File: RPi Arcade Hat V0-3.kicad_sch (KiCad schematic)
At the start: 75 parts, among them J1 Raspberry_Pi_2_3, J10 Coin/Note Input, J11 +24V IN, J12 +12V OUT, J13 Player 1, J14 Player 2, J15 Player 3, J16 Player 4, J17 ICSP, J18 Program MCU, J19 Graphics LCD, J2 Player 1, J20 Channel 4, J21 Channel 3, J22 Channel 2, J23 Channel 1, J24 CCard Input, J3 Player 2, J4 Spares, J5 Player 3, J6 Player 4, J7 +24V OUT, J8 Neo Pixel Data, J9 Note Acceptor, Q16 BC847, Q4 BC847, Q5 BC847, Q6 BC847, Q7 BC847, U1 ATmega328P-A, U2 SN74HC04N, U3 LM2595S-12, Y1 16MHz Crystal

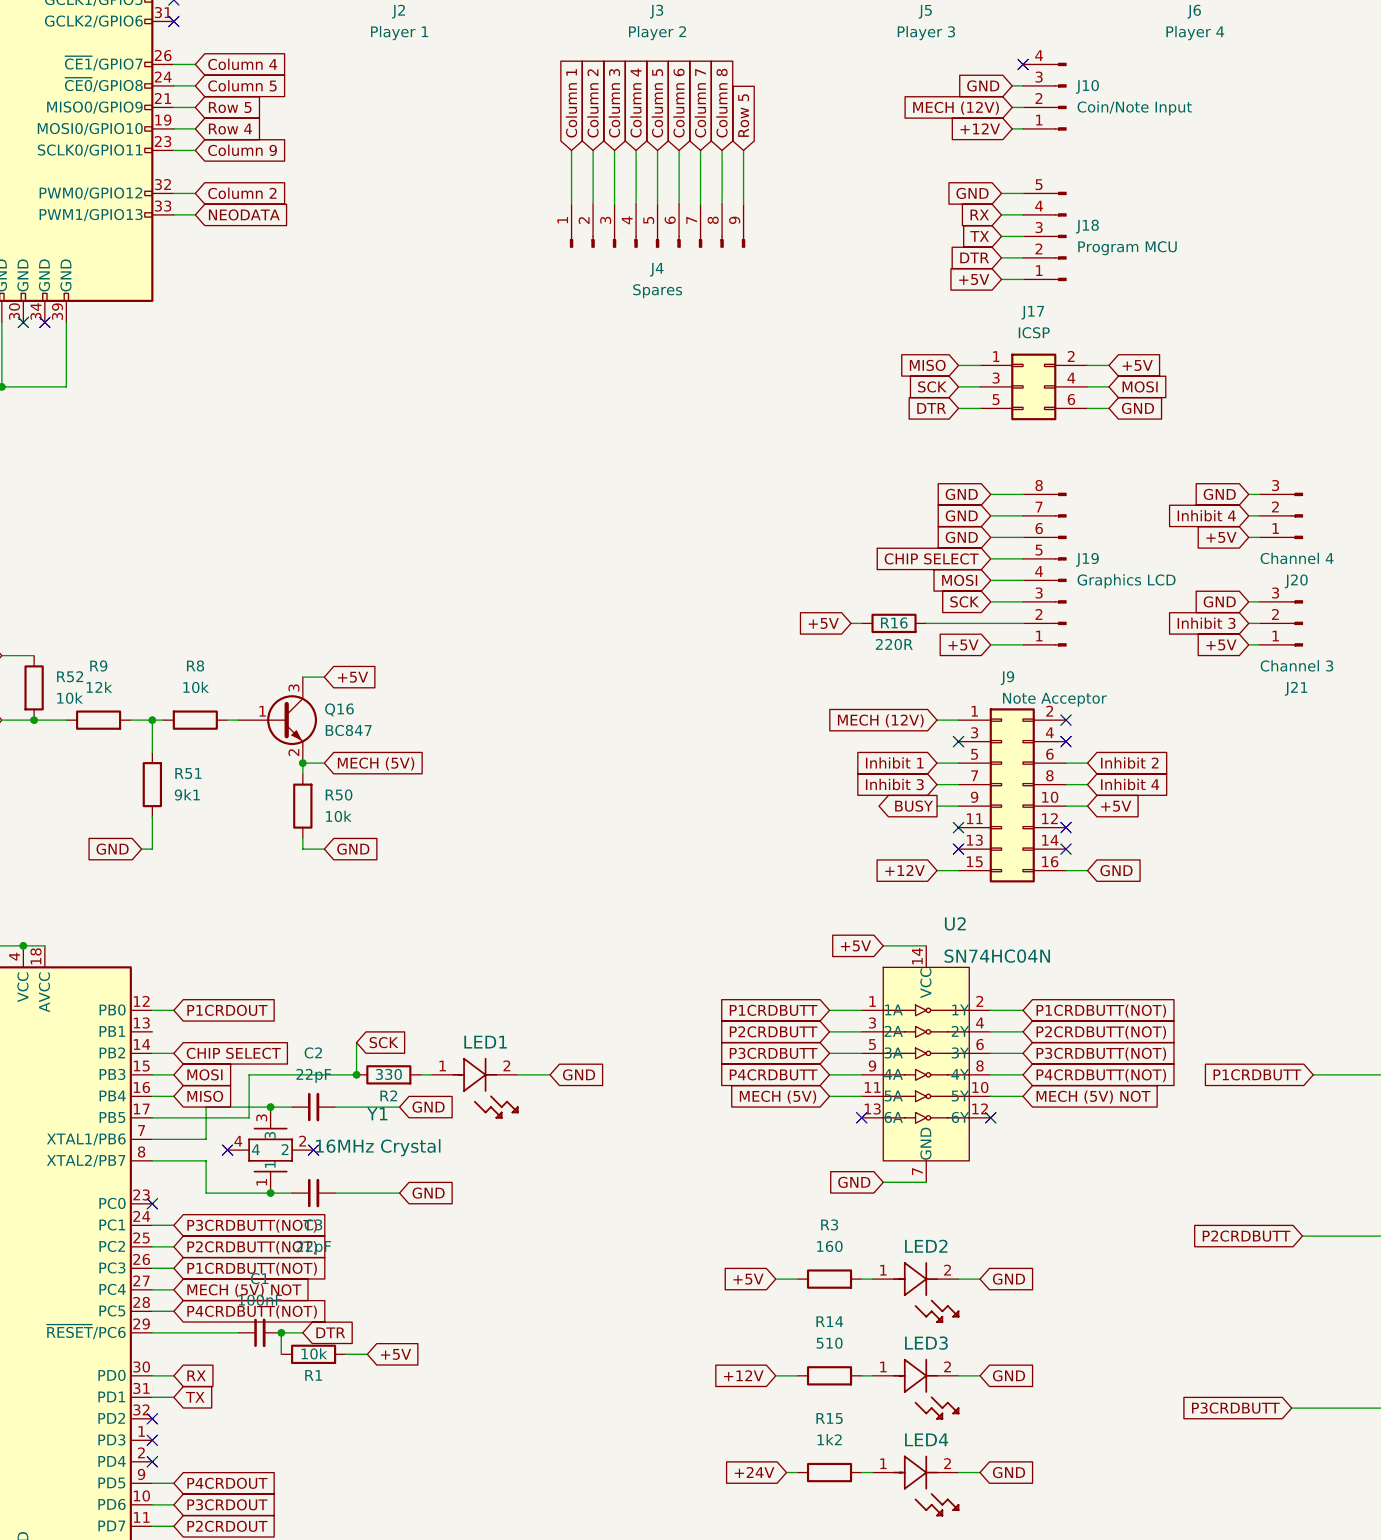
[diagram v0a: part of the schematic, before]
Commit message: Added Arduino Code
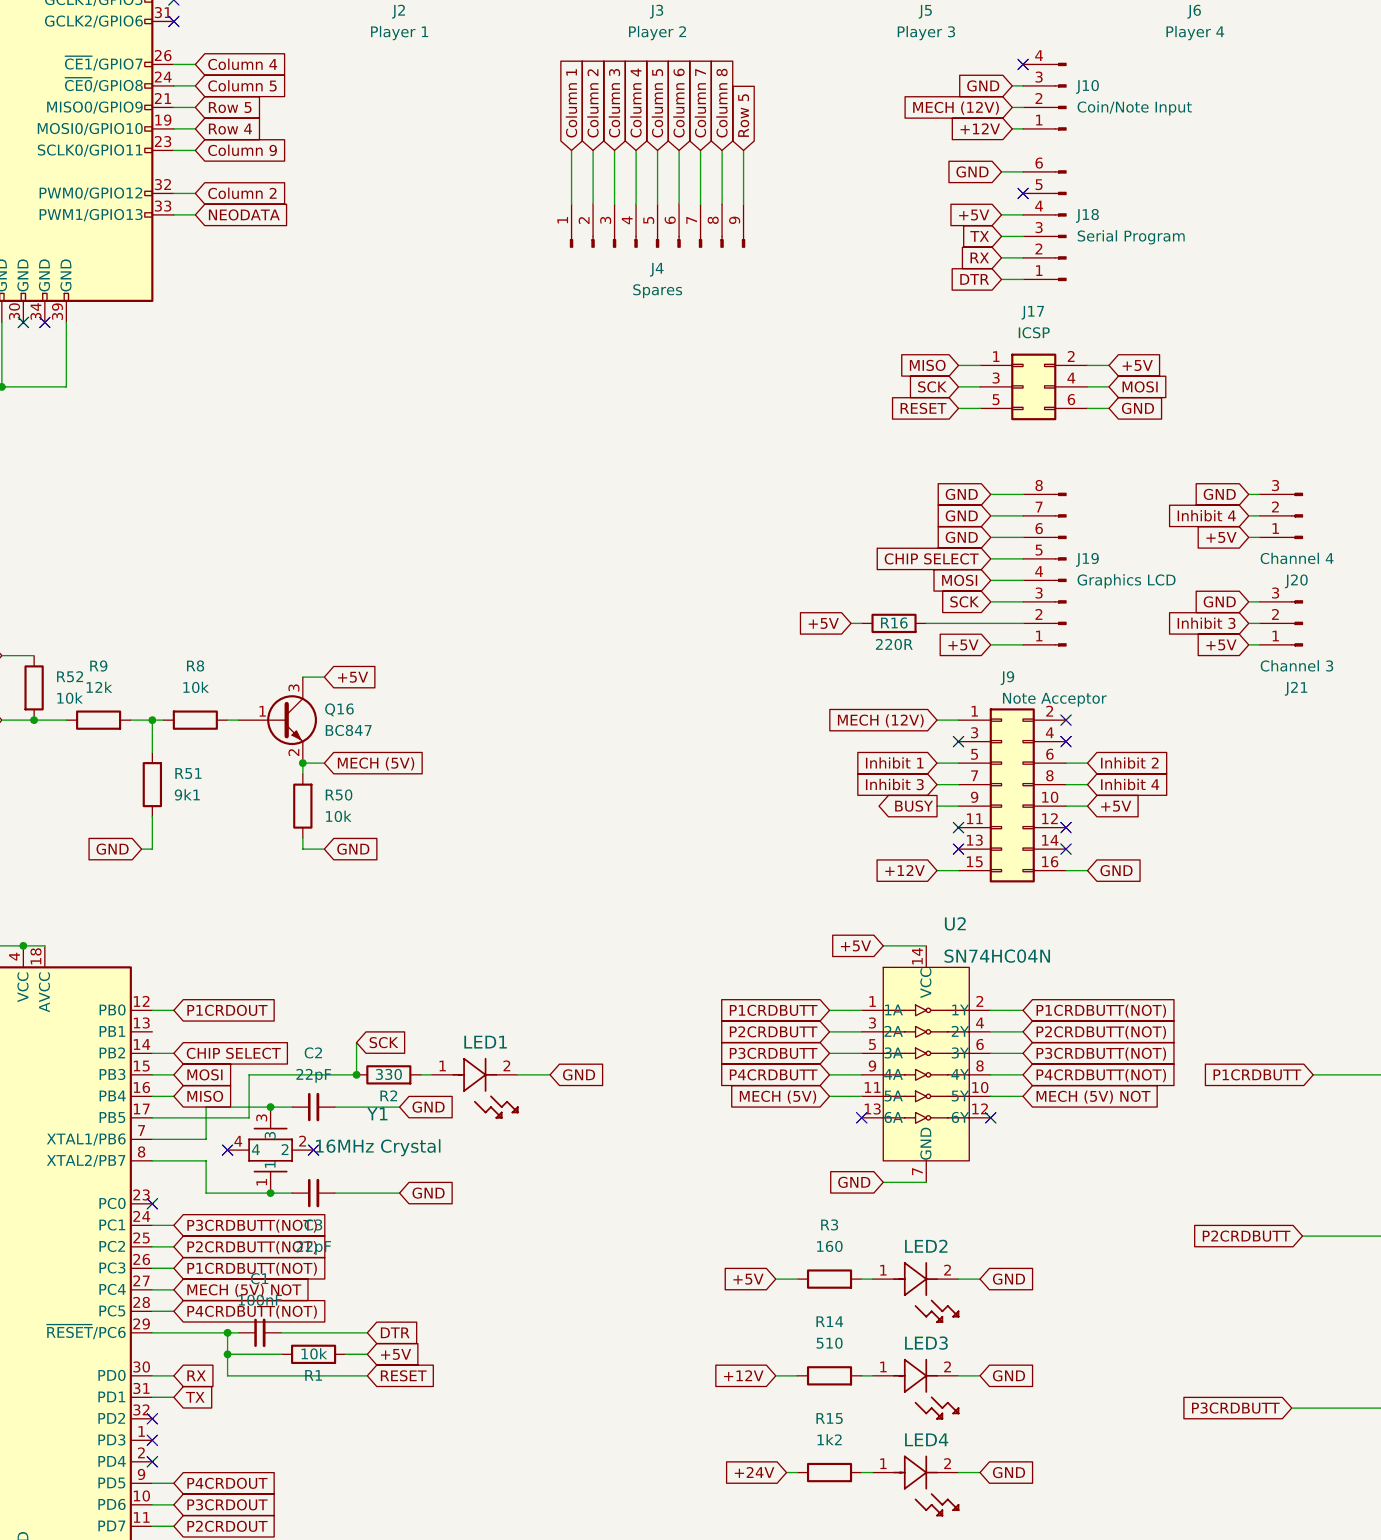
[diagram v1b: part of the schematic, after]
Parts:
- removed J18: Program MCU, Connector_PinHeader_2.54mm:PinHeader_1x05_P2.54mm_Vertical, symbol Connector:Conn_01x05_Male
- added J18: Serial Program, Connector_PinHeader_2.54mm:PinHeader_1x06_P2.54mm_Vertical, symbol Connector:Conn_01x06_Pin
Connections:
- net +5V: now also J18.4 (Pin_4)
- net DTR: now also J18.1 (Pin_1); no longer J17.5 (Pin_5), R1.1
- net GND: now also J18.6 (Pin_6)
- net RX: now also J18.2 (Pin_2)
- net TX: now also J18.3 (Pin_3)
- net RESET: now reaches C1.1, U1.29 (~{RESET}/PC6)
- net RESET: now also J17.5 (Pin_5), R1.1
- no-connect marks 36 -> 37
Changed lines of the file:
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@@
   (junction (at 63.5 257.81) (diameter 0) (color 0 0 0 0)
   )
+  (junction (at 74.93 204.47) (diameter 0) (color 0 0 0 0)
+  )
   (junction (at 83.82 137.16) (diameter 0) (color 0 0 0 0)
   )
   (junction (at 40.64 92.71) (diameter 0) (color 0 0 0 0)
   )
+  (junction (at 74.93 207.01) (diameter 0) (color 0 0 0 0)
+  )
   (junction (at 63.5 265.43) (diameter 0) (color 0 0 0 0)
   )
@@
   (junction (at 26.67 252.73) (diameter 0) (color 0 0 0 0)
   )
-  (junction (at 81.28 204.47) (diameter 0) (color 0 0 0 0)
-  )
   (junction (at 227.33 213.36) (diameter 0) (color 0 0 0 0)
   )
@@
   (no_connect (at 50.8 85.09))
   (no_connect (at 35.56 171.45))
+  (no_connect (at 168.91 69.85))
   (no_connect (at 45.72 85.09))
   (no_connect (at 161.29 134.62))
@@
     (stroke (width 0) (type default))
   )
-  (wire (pts (xy 166.37 72.39) (xy 168.91 72.39))
-    (stroke (width 0) (type default))
-  )
   (wire (pts (xy 149.86 198.12) (xy 151.13 198.12))
     (stroke (width 0) (type default))
@@
     (stroke (width 0) (type default))
   )
-  (wire (pts (xy 166.37 77.47) (xy 168.91 77.47))
-    (stroke (width 0) (type default))
-  )
   (wire (pts (xy 165.1 110.49) (xy 168.91 110.49))
     (stroke (width 0) (type default))
@@
     (stroke (width 0) (type default))
   )
+  (wire (pts (xy 74.93 209.55) (xy 74.93 207.01))
+    (stroke (width 0) (type default))
+  )
   (wire (pts (xy 248.92 190.5) (xy 247.65 190.5))
     (stroke (width 0) (type default))
   )
-  (wire (pts (xy 166.37 69.85) (xy 168.91 69.85))
+  (wire (pts (xy 166.37 67.31) (xy 168.91 67.31))
     (stroke (width 0) (type default))
   )
@@
     (stroke (width 0) (type default))
   )
+  (wire (pts (xy 74.93 204.47) (xy 76.2 204.47))
+    (stroke (width 0) (type default))
+  )
   (wire (pts (xy 147.32 34.29) (xy 147.32 40.64))
     (stroke (width 0) (type default))
@@
     (stroke (width 0) (type default))
   )
+  (wire (pts (xy 81.28 207.01) (xy 74.93 207.01))
+    (stroke (width 0) (type default))
+  )
   (wire (pts (xy 226.06 237.49) (xy 248.92 237.49))
     (stroke (width 0) (type default))
@@
     (stroke (width 0) (type default))
   )
-  (wire (pts (xy 66.04 204.47) (xy 76.2 204.47))
+  (wire (pts (xy 66.04 204.47) (xy 74.93 204.47))
     (stroke (width 0) (type default))
   )
@@
     (stroke (width 0) (type default))
   )
+  (wire (pts (xy 74.93 207.01) (xy 74.93 204.47))
+    (stroke (width 0) (type default))
+  )
   (wire (pts (xy 25.4 69.85) (xy 27.94 69.85))
     (stroke (width 0) (type default))
@@
     (stroke (width 0) (type default))
   )
+  (wire (pts (xy 166.37 74.93) (xy 168.91 74.93))
+    (stroke (width 0) (type default))
+  )
   (wire (pts (xy 231.14 171.45) (xy 231.14 173.99))
     (stroke (width 0) (type default))
@@
     (stroke (width 0) (type default))
   )
-  (wire (pts (xy 81.28 204.47) (xy 81.28 207.01))
-    (stroke (width 0) (type default))
-  )
   (wire (pts (xy 165.1 171.45) (xy 168.91 171.45))
     (stroke (width 0) (type default))
@@
     (stroke (width 0) (type default))
   )
+  (wire (pts (xy 166.37 72.39) (xy 168.91 72.39))
+    (stroke (width 0) (type default))
+  )
   (wire (pts (xy 161.29 149.86) (xy 158.75 149.86))
     (stroke (width 0) (type default))
@@
     (stroke (width 0) (type default))
   )
+  (wire (pts (xy 166.37 80.01) (xy 168.91 80.01))
+    (stroke (width 0) (type default))
+  )
   (wire (pts (xy 115.57 34.29) (xy 115.57 40.64))
     (stroke (width 0) (type default))
@@
     (stroke (width 0) (type default))
   )
-  (wire (pts (xy 66.04 166.37) (xy 68.58 166.37))
+  (wire (pts (xy 166.37 77.47) (xy 168.91 77.47))
     (stroke (width 0) (type default))
   )
-  (wire (pts (xy 166.37 80.01) (xy 168.91 80.01))
+  (wire (pts (xy 66.04 166.37) (xy 68.58 166.37))
     (stroke (width 0) (type default))
   )
@@
     (stroke (width 0) (type default))
   )
-  (wire (pts (xy 81.28 204.47) (xy 83.82 204.47))
+  (wire (pts (xy 81.28 204.47) (xy 91.44 204.47))
     (stroke (width 0) (type default))
   )
@@
     (stroke (width 0) (type default))
   )
+  (wire (pts (xy 91.44 209.55) (xy 74.93 209.55))
+    (stroke (width 0) (type default))
+  )
   (wire (pts (xy 189.23 34.29) (xy 189.23 40.64))
     (stroke (width 0) (type default))
@@
     (stroke (width 0) (type default))
   )
-  (wire (pts (xy 166.37 74.93) (xy 168.91 74.93))
-    (stroke (width 0) (type default))
-  )
   (wire (pts (xy 87.63 177.8) (xy 95.25 177.8))
     (stroke (width 0) (type default))
@@
     )
   )
-  (global_label "DTR" (shape input) (at 161.29 95.25 180) (fields_autoplaced)
+  (global_label "RESET" (shape input) (at 161.29 95.25 180) (fields_autoplaced)
     (effects (font (size 1.27 1.27)) (justify right))
-    (property "Intersheetrefs" "${INTERSHEET_REFS}" (at 155.3693 95.1706 0)
+    (property "Intersheetrefs" "${INTERSHEET_REFS}" (at 152.5597 95.25 0)
       (effects (font (size 1.27 1.27)) (justify right) hide)
     )
@@
     )
   )
-  (global_label "DTR" (shape input) (at 83.82 204.47 0) (fields_autoplaced)
+  (global_label "DTR" (shape input) (at 91.44 204.47 0) (fields_autoplaced)
     (effects (font (size 1.27 1.27)) (justify left))
-    (property "Intersheetrefs" "${INTERSHEET_REFS}" (at 89.7407 204.3906 0)
+    (property "Intersheetrefs" "${INTERSHEET_REFS}" (at 97.3607 204.3906 0)
       (effects (font (size 1.27 1.27)) (justify left) hide)
     )
@@
     )
   )
+  (global_label "RESET" (shape input) (at 91.44 209.55 0) (fields_autoplaced)
+    (effects (font (size 1.27 1.27)) (justify left))
+    (property "Intersheetrefs" "${INTERSHEET_REFS}" (at 100.1703 209.55 0)
+      (effects (font (size 1.27 1.27)) (justify left) hide)
+    )
+  )
   (global_label "Column 3" (shape input) (at 71.12 31.75 0) (fields_autoplaced)
     (effects (font (size 1.27 1.27)) (justify left))
@@
     )
   )
-  (global_label "RX" (shape input) (at 166.37 72.39 180) (fields_autoplaced)
+  (global_label "RX" (shape input) (at 166.37 77.47 180) (fields_autoplaced)
     (effects (font (size 1.27 1.27)) (justify right))
-    (property "Intersheetrefs" "${INTERSHEET_REFS}" (at 161.4774 72.3106 0)
+    (property "Intersheetrefs" "${INTERSHEET_REFS}" (at 161.4774 77.3906 0)
       (effects (font (size 1.27 1.27)) (justify right) hide)
     )
@@
     )
   )
-  (global_label "+5V" (shape input) (at 166.37 80.01 180) (fields_autoplaced)
+  (global_label "+5V" (shape input) (at 166.37 72.39 180) (fields_autoplaced)
     (effects (font (size 1.27 1.27)) (justify right))
-    (property "Intersheetrefs" "${INTERSHEET_REFS}" (at 160.0864 79.9306 0)
+    (property "Intersheetrefs" "${INTERSHEET_REFS}" (at 160.0864 72.3106 0)
       (effects (font (size 1.27 1.27)) (justify right) hide)
     )
@@
     )
   )
-  (global_label "GND" (shape input) (at 166.37 69.85 180) (fields_autoplaced)
+  (global_label "GND" (shape input) (at 166.37 67.31 180) (fields_autoplaced)
     (effects (font (size 1.27 1.27)) (justify right))
-    (property "Intersheetrefs" "${INTERSHEET_REFS}" (at 160.0864 69.7706 0)
+    (property "Intersheetrefs" "${INTERSHEET_REFS}" (at 160.0864 67.2306 0)
       (effects (font (size 1.27 1.27)) (justify right) hide)
     )
@@
     )
   )
-  (global_label "DTR" (shape input) (at 166.37 77.47 180) (fields_autoplaced)
+  (global_label "DTR" (shape input) (at 166.37 80.01 180) (fields_autoplaced)
     (effects (font (size 1.27 1.27)) (justify right))
-    (property "Intersheetrefs" "${INTERSHEET_REFS}" (at 160.4493 77.3906 0)
+    (property "Intersheetrefs" "${INTERSHEET_REFS}" (at 160.4493 79.9306 0)
       (effects (font (size 1.27 1.27)) (justify right) hide)
     )
@@
     )
   )
+  (symbol (lib_id "Connector:Conn_01x06_Pin") (at 173.99 74.93 180) (unit 1)
+    (in_bom yes) (on_board yes) (dnp no) (fields_autoplaced)
+    (property "Reference" "J18" (at 175.26 72.39 0)
+      (effects (font (size 1.27 1.27)) (justify right))
+    )
+    (property "Value" "Serial Program" (at 175.26 74.93 0)
+      (effects (font (size 1.27 1.27)) (justify right))
+    )
+    (property "Footprint" "Connector_PinHeader_2.54mm:PinHeader_1x06_P2.54mm_Vertical" (at 173.99 74.93 0)
+      (effects (font (size 1.27 1.27)) hide)
+    )
+    (property "Datasheet" "~" (at 173.99 74.93 0)
+      (effects (font (size 1.27 1.27)) hide)
+    )
+    (pin "1")
+    (pin "2")
+    (pin "3")
+    (pin "4")
+    (pin "5")
+    (pin "6")
+    (instances
+      (project "RPi Arcade Hat V0-3"
+        (path "/ad210fca-1647-45d3-94e3-209006df452e"
+          (reference "J18") (unit 1)
+        )
+      )
+    )
+  )
   (symbol (lib_id "Device:R") (at 232.41 78.74 270) (unit 1)
     (in_bom yes) (on_board yes) (dnp no)
@@
         )
       )
-    )
-  )
-  (symbol (lib_id "Connector:Conn_01x05_Male") (at 173.99 74.93 180) (unit 1)
-    (in_bom yes) (on_board yes) (dnp no) (fields_autoplaced)
-    (property "Reference" "J18" (at 175.26 73.6599 0)
-      (effects (font (size 1.27 1.27)) (justify right))
-    )
-    (property "Value" "Program MCU" (at 175.26 76.1999 0)
-      (effects (font (size 1.27 1.27)) (justify right))
-    )
-    (property "Footprint" "Connector_PinHeader_2.54mm:PinHeader_1x05_P2.54mm_Vertical" (at 173.99 74.93 0)
-      (effects (font (size 1.27 1.27)) hide)
-    )
-    (property "Datasheet" "~" (at 173.99 74.93 0)
-      (effects (font (size 1.27 1.27)) hide)
-    )
-    (pin "1")
-    (pin "2")
-    (pin "3")
-    (pin "4")
-    (pin "5")
-    (instances
-      (project "RPi Arcade Hat V0-3"
-        (path "/ad210fca-1647-45d3-94e3-209006df452e"
-          (reference "J18") (unit 1)
-        )
-      )
